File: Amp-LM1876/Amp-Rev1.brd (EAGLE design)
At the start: 92.2 x 69.3 mm, 72 parts, among them IC1 LM358N, X1 OUT, X2 IN, X3 IN, X4 AC

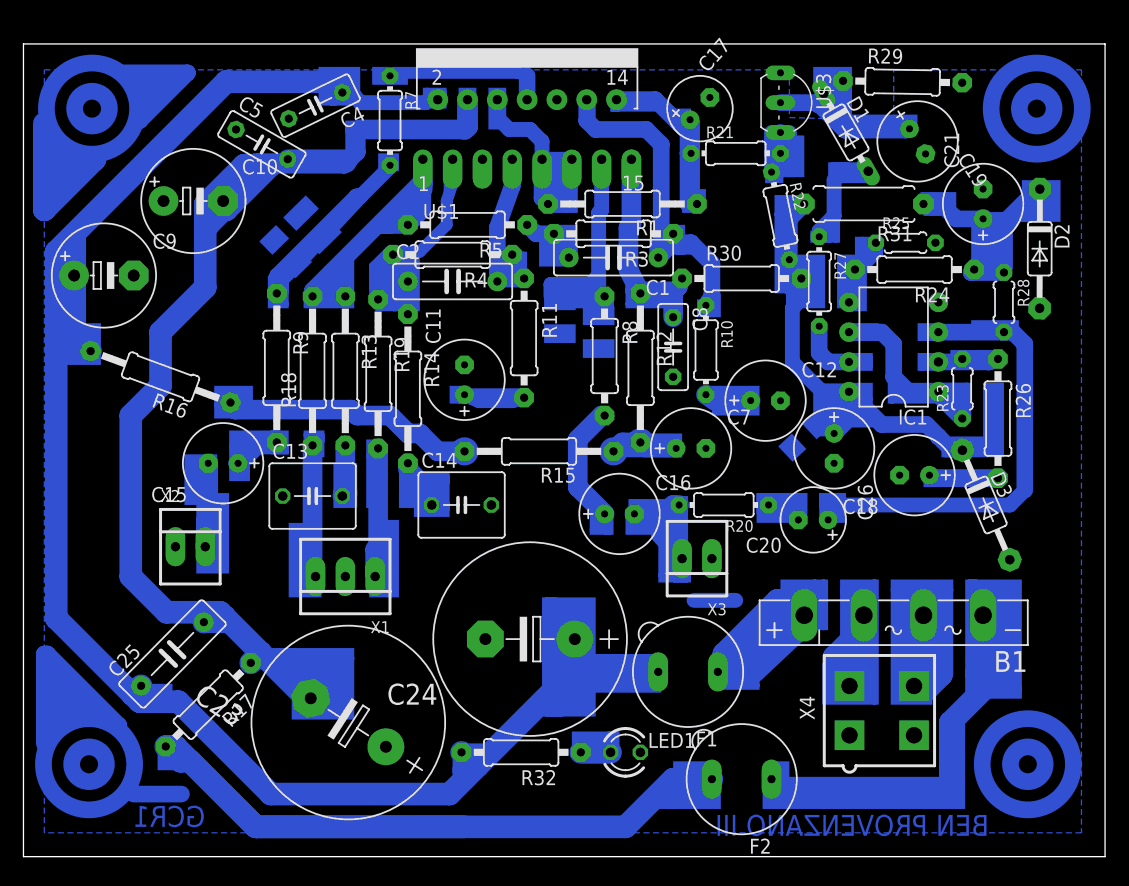
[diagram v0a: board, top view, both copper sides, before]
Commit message: 2024-11-28 10:20
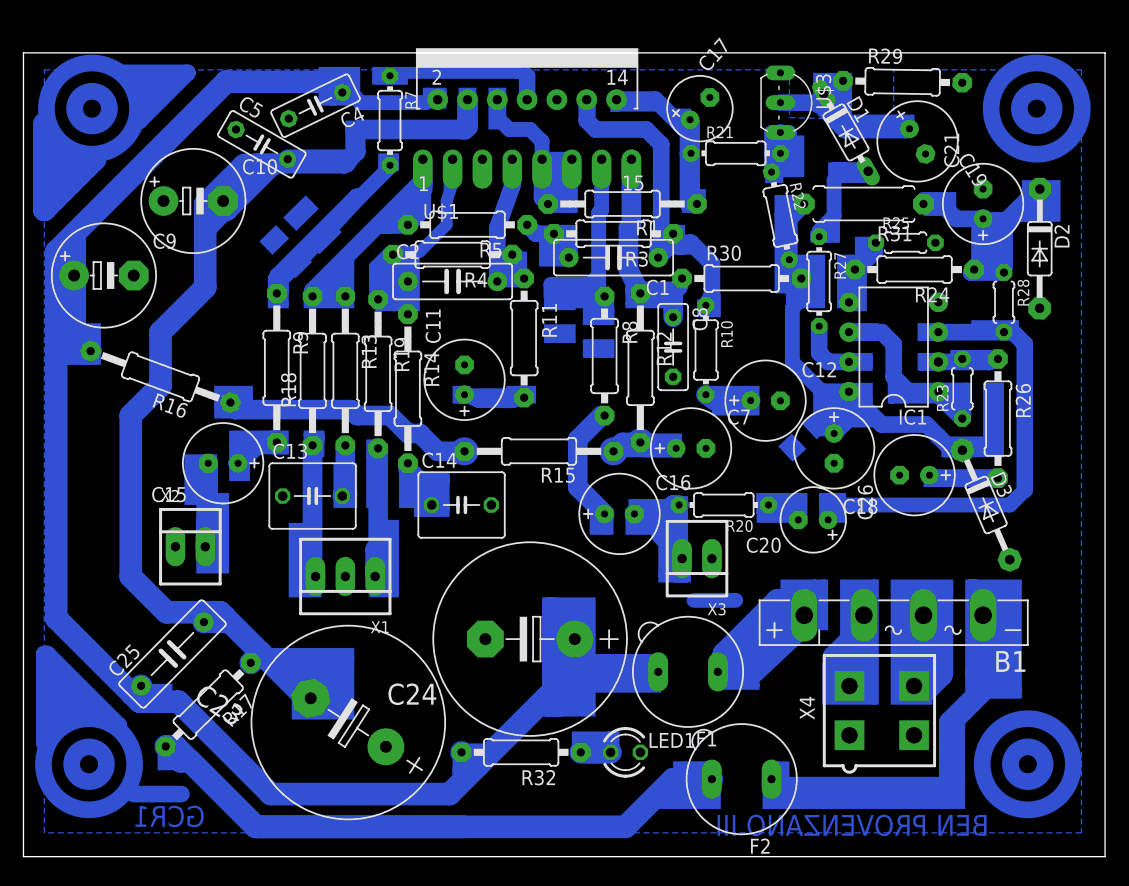
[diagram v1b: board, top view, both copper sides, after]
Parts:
- R30: value 820R -> 820R 1/2w
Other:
- board size 92.2 x 69.3 mm -> 92.2 x 68.5 mm
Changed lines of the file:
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@@
 <plain>
 <wire x1="39.624" y1="33.274" x2="131.806" y2="33.274" width="0" layer="20"/>
-<wire x1="131.806" y1="33.274" x2="131.806" y2="102.54" width="0" layer="20"/>
-<wire x1="131.806" y1="102.54" x2="39.624" y2="102.54" width="0" layer="20"/>
-<wire x1="39.624" y1="102.54" x2="39.624" y2="33.274" width="0" layer="20"/>
+<wire x1="131.806" y1="33.274" x2="131.806" y2="101.778" width="0" layer="20"/>
+<wire x1="131.806" y1="101.778" x2="39.624" y2="101.778" width="0" layer="20"/>
+<wire x1="39.624" y1="101.778" x2="39.624" y2="33.274" width="0" layer="20"/>
 <rectangle x1="65.024" y1="99.06" x2="66.548" y2="100.33" layer="16"/>
 <rectangle x1="64.77" y1="98.806" x2="65.278" y2="100.33" layer="16"/>
@@
 <rectangle x1="94.996" y1="56.642" x2="96.52" y2="58.42" layer="16"/>
 <rectangle x1="76.708" y1="71.882" x2="82.296" y2="73.152" layer="16"/>
-<rectangle x1="75.946" y1="71.882" x2="77.47" y2="73.406" layer="16"/>
+<rectangle x1="76.2" y1="71.882" x2="77.724" y2="73.406" layer="16"/>
 <rectangle x1="76.708" y1="72.39" x2="82.296" y2="73.152" layer="16"/>
 <rectangle x1="84.328" y1="84.328" x2="86.868" y2="87.122" layer="16"/>
@@
 <rectangle x1="113.284" y1="71.882" x2="113.792" y2="73.914" layer="16"/>
 <rectangle x1="113.538" y1="71.882" x2="120.142" y2="73.66" layer="16"/>
-<rectangle x1="109.728" y1="95.758" x2="115.824" y2="96.52" layer="16"/>
-<rectangle x1="106.934" y1="98.552" x2="110.236" y2="100.584" layer="16"/>
+<rectangle x1="109.474" y1="95.758" x2="115.57" y2="96.52" layer="16"/>
+<rectangle x1="106.934" y1="98.044" x2="110.236" y2="100.076" layer="16"/>
 <rectangle x1="124.714" y1="87.376" x2="128.016" y2="90.932" layer="16"/>
 <rectangle x1="123.698" y1="87.376" x2="126.238" y2="87.63" layer="16"/>
@@
 <rectangle x1="120.142" y1="70.358" x2="120.396" y2="71.12" layer="16"/>
 <rectangle x1="122.682" y1="67.31" x2="123.19" y2="73.66" layer="16"/>
+<rectangle x1="80.518" y1="72.136" x2="80.772" y2="72.39" layer="16"/>
+<rectangle x1="80.264" y1="72.136" x2="81.026" y2="72.644" layer="16"/>
+<rectangle x1="80.772" y1="72.644" x2="83.312" y2="73.406" layer="16"/>
+<rectangle x1="80.772" y1="71.882" x2="83.312" y2="72.898" layer="16"/>
 </plain>
 <attributes>
@@
 <element name="D1" library="diode" package="DO35-7" value="4148" x="109.728" y="94.996" rot="R299.9"/>
 <element name="C20" library="resistor" package="E2,5-6" value="1uF" x="106.934" y="61.976" rot="R180"/>
-<element name="R30" library="resistor" package="0207/10" value="820R" x="100.838" y="82.55"/>
+<element name="R30" library="resistor" package="0207/10" value="820R 1/2w" x="100.838" y="82.55"/>
 <element name="D2" library="diode" package="DO35-10" value="5v1" x="126.238" y="85.09" rot="R269.9"/>
 <element name="C21" library="resistor" package="E2,5-7" value="47uF" x="121.412" y="88.9" rot="R90"/>
